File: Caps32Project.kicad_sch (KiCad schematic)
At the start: 37 parts, among them J1 Ph 2.0, J2 USB_C_Receptacle_USB2.0_16P, J3 SH 1.0, Q2 AO3401A, SW1 SW_Push, SW2 SW_Push, U1 MCP73831-2-OT, U2 AP2112K-3.3, U3 ESP32-S3-WROOM-1, U4 MPU-6050

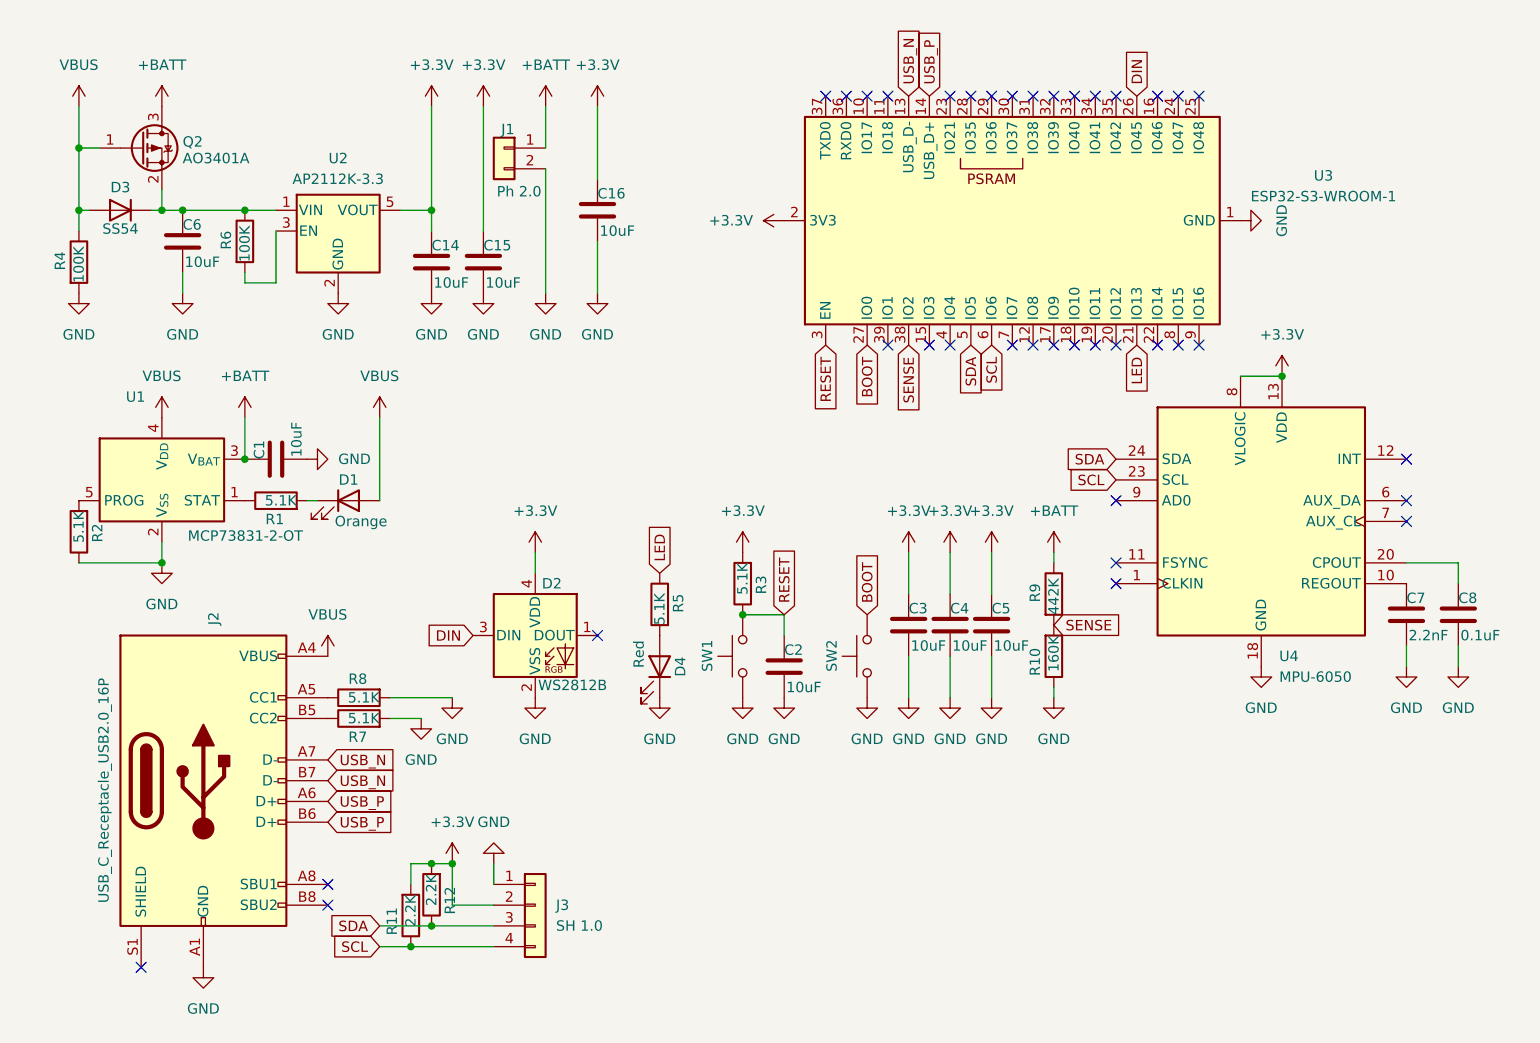
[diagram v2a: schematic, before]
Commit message: Update Board
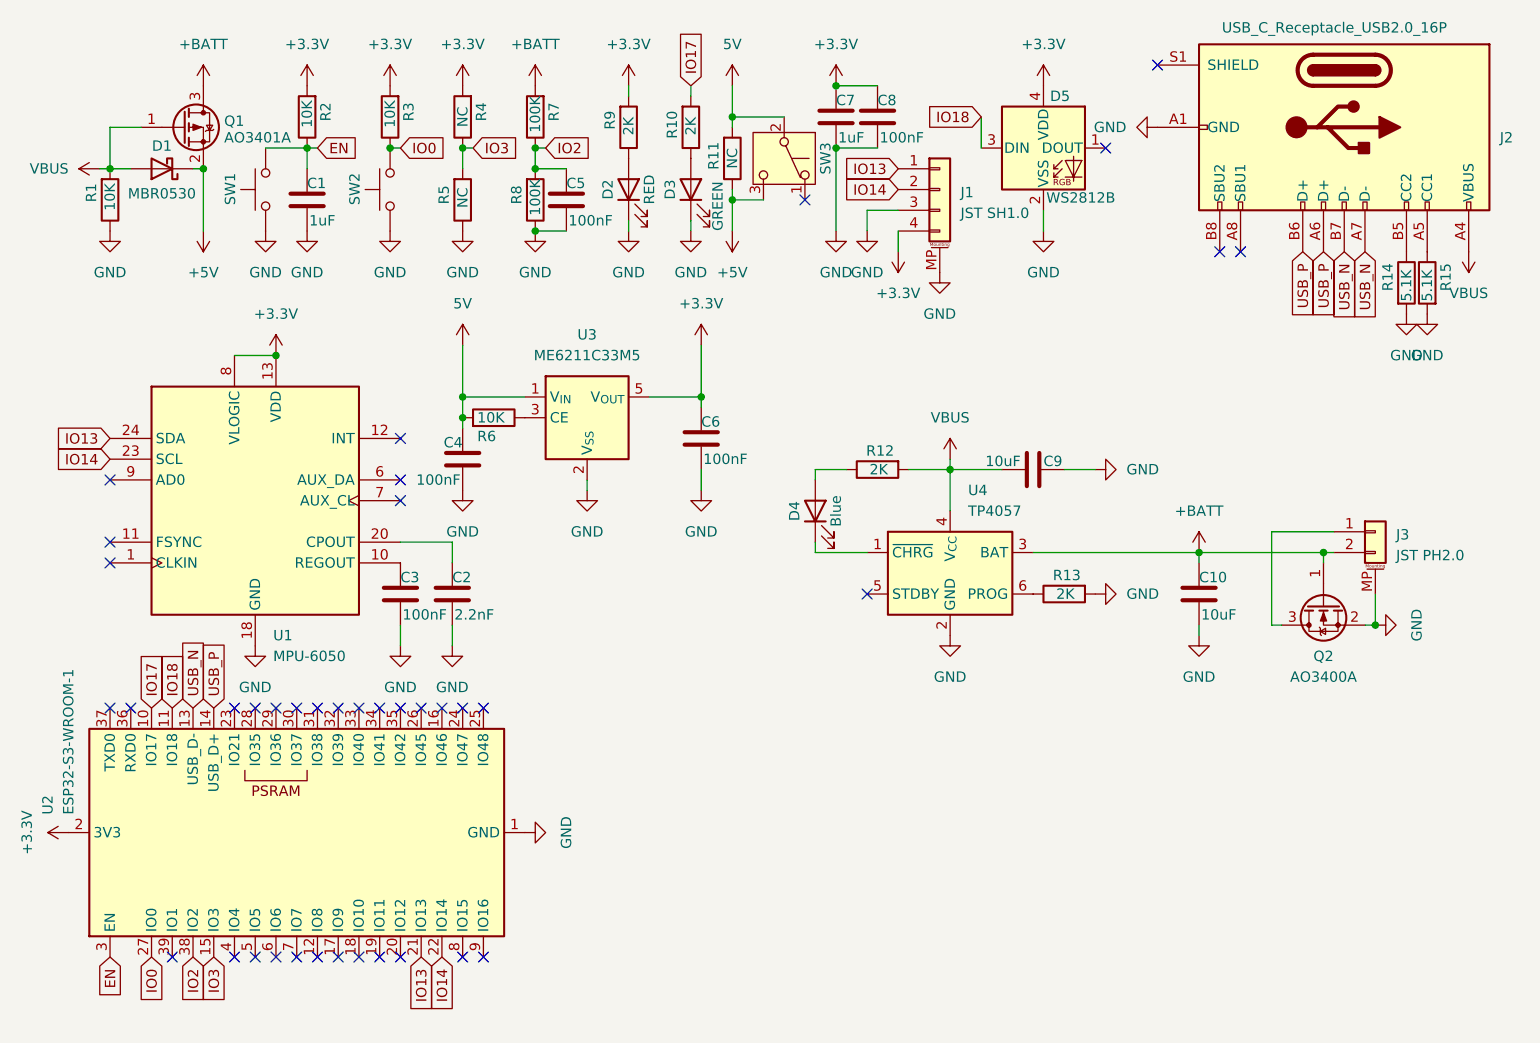
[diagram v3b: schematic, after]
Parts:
- removed C14, C15, C16: 10uF, Capacitor_SMD:C_0402_1005Metric, symbol Device:C
- removed D1: Orange, LED_SMD:LED_0402_1005Metric, symbol Device:LED
- removed D2: WS2812B, LED_SMD:LED_WS2812B-2020_PLCC4_2.0x2.0mm, symbol LED:WS2812B-2020
- removed D3: SS54, Diode_SMD:D_SMA, symbol Device:D
- removed J1: Ph 2.0, Connector_JST:JST_PH_S2B-PH-SM4-TB_1x02-1MP_P2.00mm_Horizontal, symbol Connector_Generic:Conn_01x02
- removed J3: SH 1.0, Connector_JST:JST_SH_BM04B-SRSS-TB_1x04-1MP_P1.00mm_Vertical, symbol Connector_Generic:Conn_01x04
- removed Q2: AO3401A, Package_TO_SOT_SMD:SOT-23, symbol Transistor_FET:AO3401A
- removed U1: MCP73831-2-OT, Package_TO_SOT_SMD:SOT-23-5, symbol Battery_Management:MCP73831-2-OT
- removed U2: AP2112K-3.3, Package_TO_SOT_SMD:SOT-23-5, symbol Regulator_Linear:AP2112K-3.3
- removed U3: ESP32-S3-WROOM-1, RF_Module:ESP32-S3-WROOM-1, symbol RF_Module:ESP32-S3-WROOM-1
- removed U4: MPU-6050, Sensor_Motion:InvenSense_QFN-24_4x4mm_P0.5mm, symbol Sensor_Motion:MPU-6050
- added C10, C9: 10uF, Capacitor_SMD:C_0402_1005Metric, symbol Device:C
- added D1: MBR0530, Diode_SMD:D_SOD-123, symbol Diode:MBR0530
- added D2: RED, LED_SMD:LED_0402_1005Metric, symbol Device:LED
- added D3: GREEN, LED_SMD:LED_0402_1005Metric, symbol Device:LED
- added D5: WS2812B, LED_SMD:LED_WS2812B-2020_PLCC4_2.0x2.0mm, symbol LED:WS2812B-2020
- added J1: JST SH1.0, Connector_JST:JST_SH_BM04B-SRSS-TB_1x04-1MP_P1.00mm_Vertical, symbol Connector_Generic_MountingPin:Conn_01x04_MountingPin
- added J3: JST PH2.0, Connector_JST:JST_PH_B2B-PH-SM4-TB_1x02-1MP_P2.00mm_Vertical, symbol Connector_Generic_MountingPin:Conn_01x02_MountingPin
- added Q1: AO3401A, Package_TO_SOT_SMD:SOT-23, symbol Transistor_FET:AO3401A
- added Q2: AO3400A, Package_TO_SOT_SMD:SOT-23, symbol Transistor_FET:AO3400A
- added R13: 2K, Resistor_SMD:R_0402_1005Metric, symbol Device:R
- added R14, R15: 5.1K, Resistor_SMD:R_0402_1005Metric, symbol Device:R
- added SW3: SW_Push_SPDT, Button_Switch_SMD:SW_SPDT_PCM12, symbol Switch:SW_Push_SPDT
- added U1: MPU-6050, Sensor_Motion:InvenSense_QFN-24_4x4mm_P0.5mm, symbol Sensor_Motion:MPU-6050
- added U2: ESP32-S3-WROOM-1, RF_Module:ESP32-S3-WROOM-1, symbol RF_Module:ESP32-S3-WROOM-1
- added U3: ME6211C33M5, Package_TO_SOT_SMD:SOT-23-5, symbol Regulator_Linear:ME6211C33M5
- added U4: TP4057, Package_TO_SOT_SMD:TSOT-23-6, symbol Battery_Management:TP4057
- C1: value 10uF -> 1uF
- C2: value 10uF -> 2.2nF; footprint Capacitor_SMD:C_0402_1005Metric -> Capacitor_SMD:C_0603_1608Metric
- C3, C4, C5, C6: value 10uF -> 100nF
- C7: value 2.2nF -> 1uF; footprint Capacitor_SMD:C_0603_1608Metric -> Capacitor_SMD:C_0402_1005Metric
- C8: value 0.1uF -> 100nF; footprint Capacitor_SMD:C_0201_0603Metric -> Capacitor_SMD:C_0402_1005Metric
- D4: value Red -> Blue
- J2: footprint Connector_USB:USB_C_Receptacle_GCT_USB4105-xx-A_16P_TopMnt_Horizontal -> Connector_USB:USB_C_Receptacle_GCT_USB4110
- R1, R2, R3: value 5.1K -> 10K
- R10: value 160K -> 2K; footprint Resistor_SMD:R_0805_2012Metric -> Resistor_SMD:R_0402_1005Metric
- R11: value 2.2K -> NC
- R12: value 2.2K -> 2K
- R4: value 100K -> NC; footprint Resistor_SMD:R_0201_0603Metric -> Resistor_SMD:R_0402_1005Metric
- R5: value 5.1K -> NC
- R6: value 100K -> 10K; footprint Resistor_SMD:R_0201_0603Metric -> Resistor_SMD:R_0402_1005Metric
- R7, R8: value 5.1K -> 100K
- R9: value 442K -> 2K; footprint Resistor_SMD:R_0805_2012Metric -> Resistor_SMD:R_0402_1005Metric
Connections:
- net LED is gone; now on net GND: R5.1
- net SDA is gone; now on an unnamed net: R12.1
- net +3.3V: now also C6.1, C7.1, C8.1, R2.2, R4.2, R9.2, D5.4 (VDD), J1.4 (Pin_4), U1.13 (VDD), U1.8 (VLOGIC), U2.2 (3V3), U3.5 (V_{OUT}); no longer C3.1, C4.1, C5.1, R11.2, R12.2
- net +BATT: now also R7.2, C10.1, J3.2 (Pin_2), Q1.3 (D), Q2.1 (G), U4.3 (BAT); no longer C1.1, R9.1
- net GND: now also R1.1, R8.1, C10.2, C9.1, D2.1 (K), D3.1 (K), D5.2 (VSS), J1.3 (Pin_3), J1.MP (MountPin), J3.MP (MountPin), Q2.2 (S), R13.2, R14.2, R15.2, U1.18 (GND), U2.1 (GND), U2.40 (GND), U2.41 (GND), U3.2 (V_{SS}), U4.2 (GND); no longer D4.1 (K), R10.1, R2.1, R4.2, R7.2, R8.2
- net USB_N: now also U2.13 (USB_D-)
- net USB_P: now also U2.14 (USB_D+)
- net VBUS: now also R1.2, R12.2, C9.2, D1.2 (A), Q1.1 (G), U4.4 (V_{CC}); no longer R4.1
- net at J2.B5 (CC2): now also R14.1; no longer R7.1
- net at J2.A5 (CC1): now also R15.1; no longer R8.1
- net at R6.1: now also U3.3 (CE); no longer C6.1
- net 5V: now reaches R6.2
- net 5V: now also C4.1, R11.2, SW3.2 (B), U3.1 (V_{IN})
- net at D4.2 (A): no longer R5.2
- net BOOT renamed IO0
- net IO0: now also R3.1, U2.27 (IO0)
- removed net RESET: C2.1, R3.1, SW1.2
- net SCL renamed +5V
- net +5V: now also D1.1 (K), Q1.2 (S), SW3.3 (C)
- net SENSE renamed IO17
- net IO17: now also U2.10 (IO17); no longer R9.2
- new net: D3.2 (A), R10.1
- new net: D2.2 (A), R9.1
- new net: R13.1, U4.6 (PROG)
- new net: C3.1, U1.10 (REGOUT)
- new net: D4.1 (K), U4.1 (~{CHRG})
- new net: J3.1 (Pin_1), Q2.3 (D)
- new net: C2.1, U1.20 (CPOUT)
- new net EN: C1.1, R2.1, SW1.2, U2.3 (EN)
- new net IO13: J1.1 (Pin_1), U1.24 (SDA), U2.21 (IO13)
- new net IO14: J1.2 (Pin_2), U1.23 (SCL), U2.22 (IO14)
- new net IO18: D5.3 (DIN), U2.11 (IO18)
- new net IO2: C5.1, R7.1, R8.2, U2.38 (IO2)
- new net IO3: R4.1, R5.2, U2.15 (IO3)
- no-connect marks 38 -> 39

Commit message: Update Board
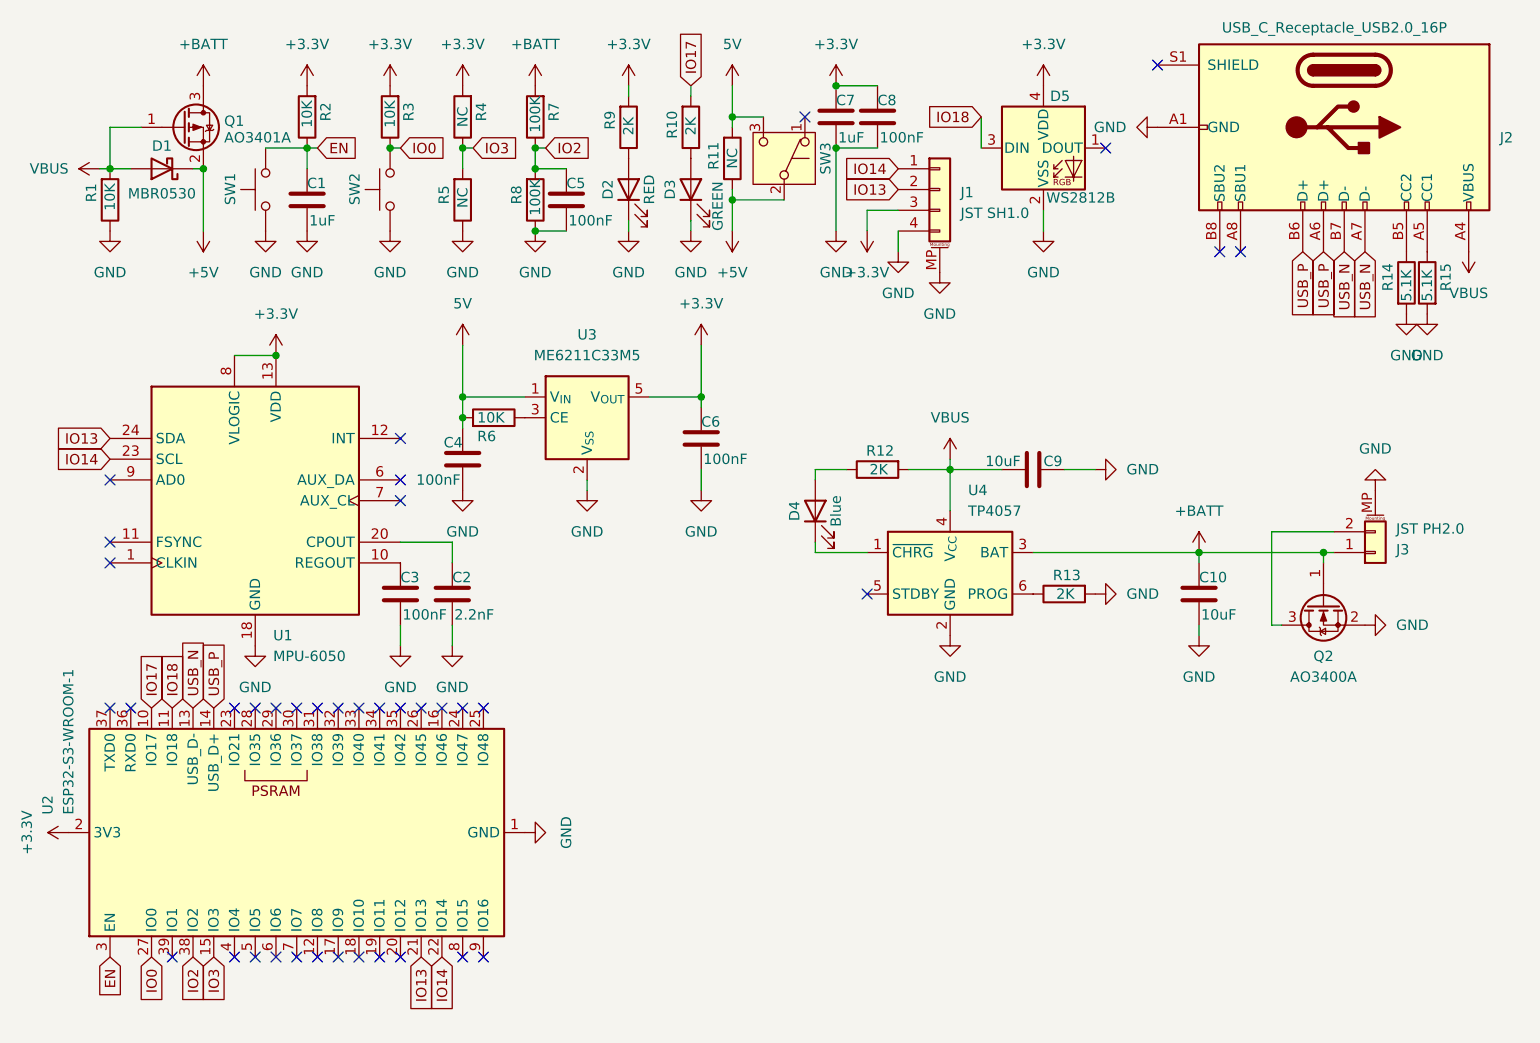
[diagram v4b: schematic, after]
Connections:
- net +3.3V: now also J1.3 (Pin_3); no longer J1.4 (Pin_4)
- net +5V: now also SW3.2 (B); no longer SW3.3 (C)
- net +BATT: now also J3.1 (Pin_1); no longer J3.2 (Pin_2)
- net 5V: now also SW3.3 (C); no longer SW3.2 (B)
- net GND: now also J1.4 (Pin_4); no longer J1.3 (Pin_3)
- net IO13: now also J1.2 (Pin_2); no longer J1.1 (Pin_1)
- net IO14: now also J1.1 (Pin_1); no longer J1.2 (Pin_2)
- net at Q2.3 (D): now also J3.2 (Pin_2); no longer J3.1 (Pin_1)

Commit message: Update Board
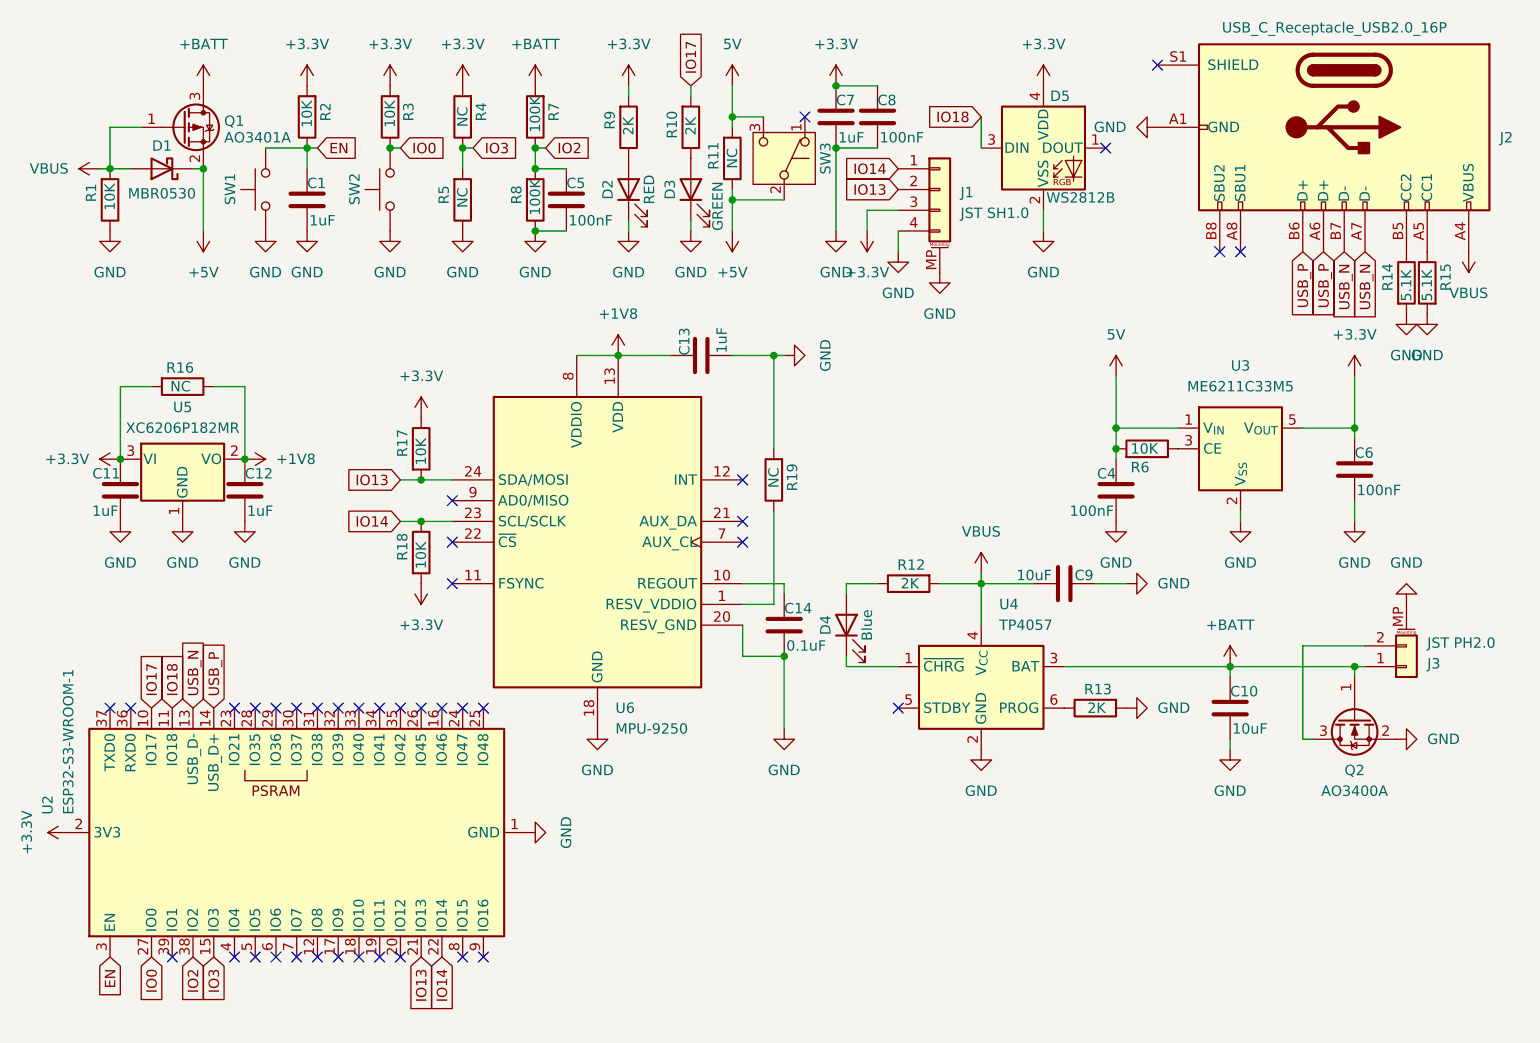
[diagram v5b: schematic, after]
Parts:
- removed C2: 2.2nF, Capacitor_SMD:C_0603_1608Metric, symbol Device:C
- removed C3: 100nF, Capacitor_SMD:C_0402_1005Metric, symbol Device:C
- removed U1: MPU-6050, Sensor_Motion:InvenSense_QFN-24_4x4mm_P0.5mm, symbol Sensor_Motion:MPU-6050
- added C11, C12, C13: 1uF, Capacitor_SMD:C_0402_1005Metric, symbol Device:C
- added C14: 0.1uF, Capacitor_SMD:C_0402_1005Metric, symbol Device:C
- added R16, R19: NC, Resistor_SMD:R_0402_1005Metric, symbol Device:R
- added R17, R18: 10K, Resistor_SMD:R_0402_1005Metric, symbol Device:R
- added U5: XC6206P182MR, Package_TO_SOT_SMD:SOT-23-3, symbol Regulator_Linear:XC6206PxxxMR
- added U6: MPU-9250, Sensor_Motion:InvenSense_QFN-24_3x3mm_P0.4mm, symbol Sensor_Motion:MPU-9250
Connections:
- net +3.3V: now also C11.1, R16.2, R17.1, R18.2, U5.3 (VI)
- net GND: now also C11.2, C12.2, C13.2, C14.2, R19.2, U5.1 (GND), U6.18 (GND), U6.20 (RESV_GND)
- net IO13: now also R17.2, U6.24 (SDA/MOSI)
- net IO14: now also R18.1, U6.23 (SCL/SCLK)
- new net: C14.1, U6.10 (REGOUT)
- new net: R19.1, U6.1 (RESV_VDDIO)
- new net +1V8: C12.1, C13.1, R16.1, U5.2 (VO), U6.13 (VDD), U6.8 (VDDIO)
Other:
- moved on the sheet: C10, C4, C6, C9, D4, J3, Q2, R12, R13, R6, U3, U4
